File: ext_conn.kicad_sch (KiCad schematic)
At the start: 4 parts

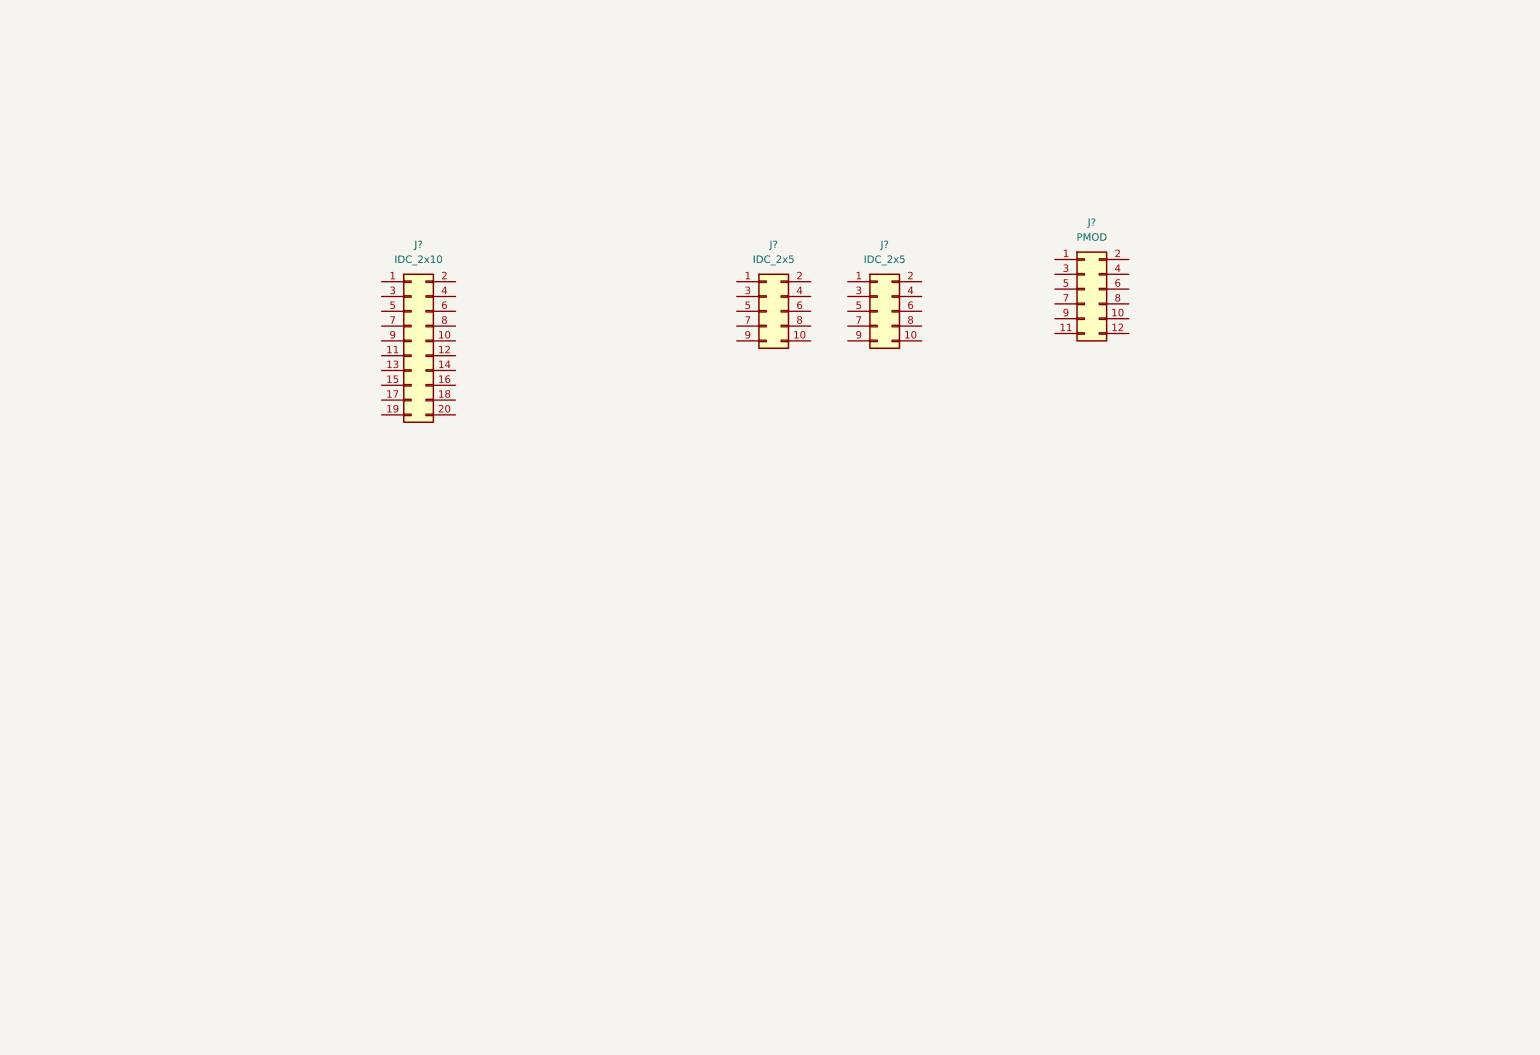
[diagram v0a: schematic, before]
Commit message: schematic almost done
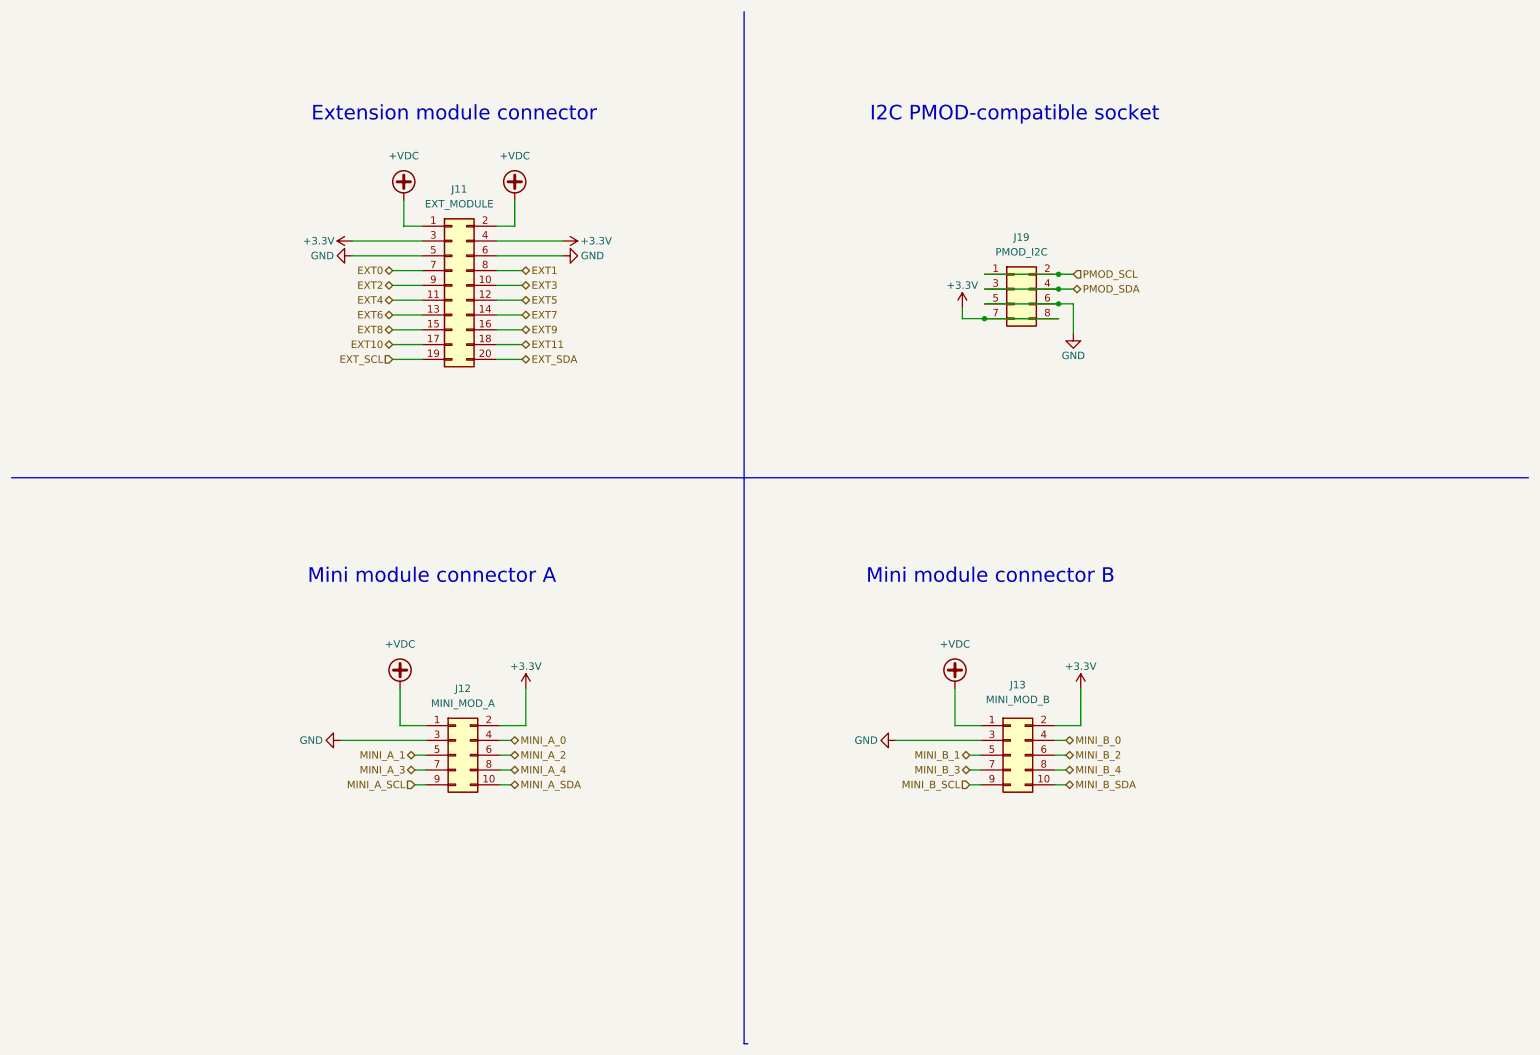
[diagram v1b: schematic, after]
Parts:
- removed J?: PMOD, Connector_PinSocket_2.54mm:PinSocket_2x06_P2.54mm_Vertical, symbol Connector_Generic:Conn_02x06_Odd_Even
- removed J?: IDC_2x5, Connector_IDC:IDC-Header_2x05_P2.54mm_Vertical, symbol Connector_Generic:Conn_02x05_Odd_Even
- added J13: MINI_MOD_B, Connector_IDC:IDC-Header_2x05_P2.54mm_Vertical, symbol Connector_Generic:Conn_02x05_Odd_Even
- added J19: PMOD_I2C, Connector_PinSocket_2.54mm:PinSocket_2x04_P2.54mm_Vertical, symbol Connector_Generic:Conn_02x04_Odd_Even
- J11: renamed from J?; value IDC_2x10 -> EXT_MODULE
- J12: renamed from J?; value IDC_2x5 -> MINI_MOD_A
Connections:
- net +VDC: now reaches J11.1 (Pin_1)
- net +VDC: now also J11.2 (Pin_2), J12.1 (Pin_1), J13.1 (Pin_1)
- net EXT3: now reaches J11.10 (Pin_10)
- net EXT4: now reaches J11.11 (Pin_11)
- net EXT5: now reaches J11.12 (Pin_12)
- net EXT6: now reaches J11.13 (Pin_13)
- net EXT7: now reaches J11.14 (Pin_14)
- net EXT8: now reaches J11.15 (Pin_15)
- net EXT9: now reaches J11.16 (Pin_16)
- net EXT10: now reaches J11.17 (Pin_17)
- net EXT11: now reaches J11.18 (Pin_18)
- net EXT_SCL: now reaches J11.19 (Pin_19)
- net EXT_SDA: now reaches J11.20 (Pin_20)
- net +3V3: now reaches J11.3 (Pin_3)
- net +3V3: now also J11.4 (Pin_4), J12.2 (Pin_2), J13.2 (Pin_2), J19.7 (Pin_7), J19.8 (Pin_8)
- net GND: now reaches J11.5 (Pin_5)
- net GND: now also J11.6 (Pin_6), J12.3 (Pin_3), J13.3 (Pin_3), J19.5 (Pin_5), J19.6 (Pin_6)
- net EXT0: now reaches J11.7 (Pin_7)
- net EXT1: now reaches J11.8 (Pin_8)
- net EXT2: now reaches J11.9 (Pin_9)
- net MINI_A_SDA: now reaches J12.10 (Pin_10)
- net MINI_A_0: now reaches J12.4 (Pin_4)
- net MINI_A_1: now reaches J12.5 (Pin_5)
- net MINI_A_2: now reaches J12.6 (Pin_6)
- net MINI_A_3: now reaches J12.7 (Pin_7)
- net MINI_A_4: now reaches J12.8 (Pin_8)
- net MINI_A_SCL: now reaches J12.9 (Pin_9)
- new net MINI_B_0: J13.4 (Pin_4)
- new net MINI_B_1: J13.5 (Pin_5)
- new net MINI_B_2: J13.6 (Pin_6)
- new net MINI_B_3: J13.7 (Pin_7)
- new net MINI_B_4: J13.8 (Pin_8)
- new net MINI_B_SCL: J13.9 (Pin_9)
- new net MINI_B_SDA: J13.10 (Pin_10)
- new net PMOD_SCL: J19.1 (Pin_1), J19.2 (Pin_2)
- new net PMOD_SDA: J19.3 (Pin_3), J19.4 (Pin_4)
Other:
- note added: "Extension module connector"
- note added: "I2C PMOD-compatible socket"
- note added: "Mini module connector A"
- note added: "Mini module connector B"
- moved on the sheet: J11, J12
